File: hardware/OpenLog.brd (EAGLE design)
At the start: 17.8 x 19.1 mm, 20 parts, among them Q1 16MHZ, U1 ATMEGA328P_TQFP, U2 3.3V MIC5205, U3 microSD Socket

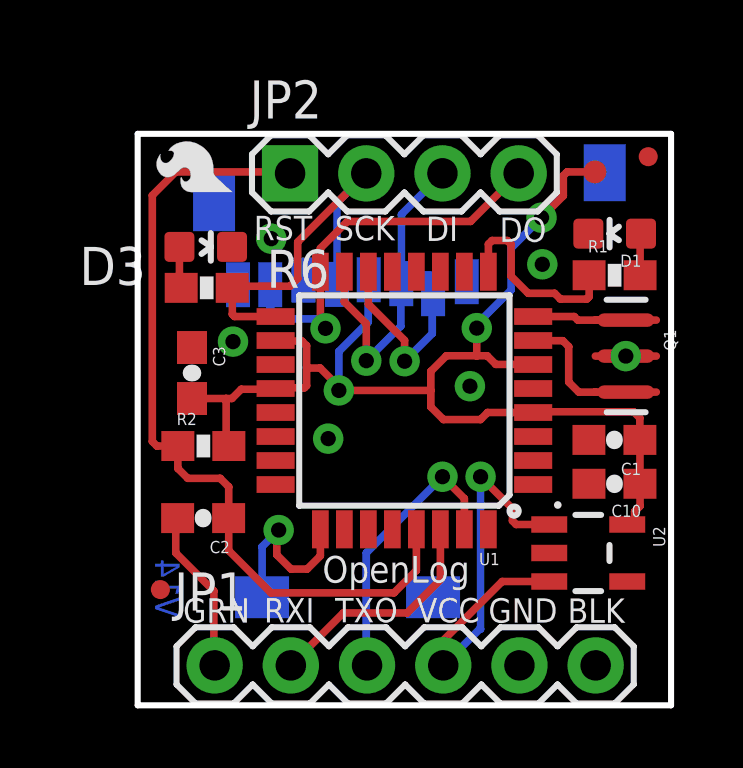
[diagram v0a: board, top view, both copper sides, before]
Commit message: Headers moved on grid.
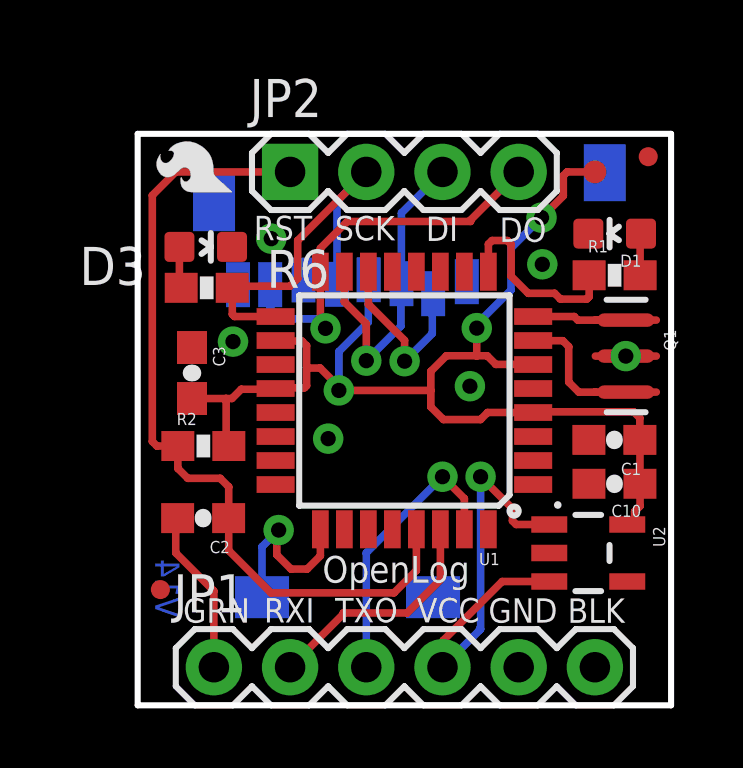
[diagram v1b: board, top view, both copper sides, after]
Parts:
- moved JP1 0.07 mm to (21.6, -8.89)
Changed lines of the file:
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@@
 <setting verticaltext="up"/>
 </settings>
-<grid distance="0.05" unitdist="inch" unit="inch" style="lines" multiple="1" display="yes" altdistance="0.0001" altunitdist="inch" altunit="inch"/>
+<grid distance="0.05" unitdist="inch" unit="inch" style="lines" multiple="1" display="yes" altdistance="0.005" altunitdist="inch" altunit="inch"/>
 <layers>
 <layer number="1" name="Top" color="4" fill="1" visible="yes" active="yes"/>
@@
 <layer number="47" name="Measures" color="7" fill="1" visible="no" active="yes"/>
 <layer number="48" name="Document" color="7" fill="1" visible="no" active="yes"/>
-<layer number="49" name="Reference" color="7" fill="1" visible="yes" active="yes"/>
+<layer number="49" name="Reference" color="7" fill="1" visible="no" active="yes"/>
 <layer number="50" name="dxf" color="7" fill="1" visible="no" active="yes"/>
 <layer number="51" name="tDocu" color="6" fill="1" visible="yes" active="yes"/>
@@
 <attribute name="PROD_ID" value="XTAL-08900" x="35.321240625" y="1.48081875" size="1.778" layer="27" rot="R270" display="off"/>
 </element>
-<element name="JP1" library="SparkFun" package="1X06" value="Serial Connection" x="21.6154" y="-8.8290375"/>
+<element name="JP1" library="SparkFun" package="1X06" value="Serial Connection" x="21.59" y="-8.89"/>
 <element name="C2" library="SparkFun-Capacitors" package="0603-CAP" value="0.1uF" x="21.231859375" y="-3.919221875" rot="R180">
 <attribute name="PROD_ID" value="CAP-00810" x="21.231859375" y="-3.919221875" size="1.778" layer="27" rot="R180" display="off"/>
@@
 <attribute name="VALUE" value="1.0uF" x="34.9402375" y="-1.313175" size="1.778" layer="27" rot="R180" display="off"/>
 </element>
-<element name="JP2" library="SparkFun" package="1X04" value="" x="24.13" y="7.571740625"/>
+<element name="JP2" library="SparkFun" package="1X04" value="" x="24.13" y="7.62"/>
 <element name="U1" library="SparkFun-DigitalIC" package="TQFP32-08" value="ATMEGA328P_TQFP" x="27.94" y="0" rot="R180">
 <attribute name="PROD_ID" value="IC-09069" x="27.94" y="0" size="0.8128" layer="27" font="vector" ratio="15" rot="R180" display="off"/>
@@
 <contactref element="U1" pad="17"/>
 <wire x1="22.204678125" y1="3.753225" x2="22.201240625" y2="3.7566625" width="0.254" layer="1"/>
-<wire x1="25.69464375" y1="3.870953125" x2="25.69464375" y2="6.596384375" width="0.254" layer="16"/>
-<wire x1="25.69464375" y1="6.596384375" x2="26.67" y2="7.571740625" width="0.254" layer="16"/>
-<wire x1="24.384" y1="4.064" x2="24.384" y2="5.285740625" width="0.254" layer="1"/>
-<wire x1="24.384" y1="5.285740625" x2="26.67" y2="7.571740625" width="0.254" layer="1"/>
+<wire x1="25.69464375" y1="3.870953125" x2="25.69464375" y2="6.64464375" width="0.254" layer="16"/>
+<wire x1="24.384" y1="4.064" x2="24.384" y2="5.334" width="0.254" layer="1"/>
 <wire x1="23.6474" y1="2.8" x2="22.2799625" y2="2.8" width="0.254" layer="1"/>
 <wire x1="22.2799625" y1="2.8" x2="22.20468125" y2="2.87528125" width="0.254" layer="1"/>
@@
 <wire x1="24.13" y1="3.81" x2="22.254578125" y2="3.81" width="0.254" layer="1"/>
 <wire x1="22.254578125" y1="3.81" x2="22.201240625" y2="3.7566625" width="0.254" layer="1"/>
+<wire x1="24.384" y1="5.334" x2="26.67" y2="7.62" width="0.254" layer="1"/>
+<wire x1="25.69464375" y1="6.64464375" x2="26.67" y2="7.62" width="0.254" layer="16"/>
 </signal>
 <signal name="MISO">
@@
 <contactref element="U1" pad="16"/>
 <wire x1="25.14" y1="5.074" x2="25.14" y2="4.2926" width="0.254" layer="1"/>
-<wire x1="30.147259375" y1="5.969" x2="31.75" y2="7.571740625" width="0.254" layer="1"/>
 <wire x1="23.45181875" y1="3.086103125" x2="23.815040625" y2="2.72288125" width="0.254" layer="16"/>
 <wire x1="23.815040625" y1="2.72288125" x2="24.99360625" y2="2.72288125" width="0.254" layer="16"/>
@@
 <wire x1="23.45181875" y1="3.086103125" x2="23.45181875" y2="3.846415625" width="0.254" layer="16"/>
 <wire x1="23.45181875" y1="3.846415625" x2="23.4672125" y2="3.861809375" width="0.254" layer="16"/>
+<wire x1="30.147259375" y1="5.969" x2="30.147259375" y2="6.017259375" width="0.254" layer="1"/>
+<wire x1="30.147259375" y1="6.017259375" x2="31.75" y2="7.62" width="0.254" layer="1"/>
 </signal>
 <signal name="MOSI">
@@
 <wire x1="27.82149375" y1="2.479915625" x2="27.82149375" y2="3.876034375" width="0.254" layer="16"/>
 <wire x1="27.82149375" y1="3.876034375" x2="27.8418125" y2="3.896353125" width="0.254" layer="16"/>
-<wire x1="27.8418125" y1="3.896353125" x2="27.8418125" y2="6.203553125" width="0.254" layer="16"/>
-<wire x1="27.8418125" y1="6.203553125" x2="29.21" y2="7.571740625" width="0.254" layer="16"/>
+<wire x1="27.8418125" y1="3.896353125" x2="27.8418125" y2="6.2518125" width="0.254" layer="16"/>
+<wire x1="27.8418125" y1="6.2518125" x2="29.21" y2="7.62" width="0.254" layer="16"/>
 </signal>
 <signal name="N$7">
@@
 <contactref element="U1" pad="31"/>
 <wire x1="29.94" y1="-3.27" x2="29.94" y2="-4.2926" width="0.254" layer="1"/>
-<wire x1="26.67" y1="-5.08" x2="26.67" y2="-8.8036375" width="0.254" layer="16"/>
-<wire x1="26.67" y1="-8.8036375" x2="26.6954" y2="-8.8290375" width="0.254" layer="16"/>
+<wire x1="26.67" y1="-5.08" x2="26.67" y2="-8.89" width="0.254" layer="16"/>
 </signal>
 <signal name="RAW" class="1">
@@
 <wire x1="31.54171875" y1="-3.60171875" x2="30.48" y2="-2.54" width="0.254" layer="1"/>
 <wire x1="30.48" y1="-7.62" x2="30.4444375" y2="-7.62" width="0.254" layer="16"/>
-<wire x1="30.4444375" y1="-7.62" x2="29.2354" y2="-8.8290375" width="0.254" layer="16"/>
-<wire x1="29.2354" y1="-8.8290375" x2="29.2354" y2="-7.99591875" width="0.254" layer="1"/>
 <wire x1="29.2354" y1="-7.99591875" x2="31.19881875" y2="-6.0325" width="0.254" layer="1"/>
 <wire x1="31.19881875" y1="-6.0325" x2="32.76888125" y2="-6.0325" width="0.254" layer="1"/>
 <wire x1="32.76888125" y1="-6.0325" x2="32.768921875" y2="-6.032540625" width="0.254" layer="1"/>
+<wire x1="29.2354" y1="-7.99591875" x2="29.2354" y2="-8.8646" width="0.254" layer="1"/>
+<wire x1="29.2354" y1="-8.8646" x2="29.21" y2="-8.89" width="0.254" layer="1"/>
+<wire x1="30.4444375" y1="-7.62" x2="30.4444375" y2="-7.6555625" width="0.254" layer="16"/>
+<wire x1="30.4444375" y1="-7.6555625" x2="29.21" y2="-8.89" width="0.254" layer="16"/>
 </signal>
 <signal name="N$1">
@@
 <wire x1="20.32" y1="-5.08" x2="20.32" y2="-3.98108125" width="0.254" layer="1"/>
 <wire x1="20.32" y1="-3.98108125" x2="20.381859375" y2="-3.919221875" width="0.254" layer="1"/>
-<wire x1="21.59" y1="-6.35" x2="21.59" y2="-8.8036375" width="0.254" layer="1"/>
-<wire x1="21.59" y1="-8.8036375" x2="21.6154" y2="-8.8290375" width="0.254" layer="1"/>
+<wire x1="21.59" y1="-6.35" x2="21.59" y2="-8.89" width="0.254" layer="1"/>
 </signal>
 <signal name="RXI">
@@
 <wire x1="29.14" y1="-5.9780375" x2="28.03651875" y2="-7.08151875" width="0.254" layer="1"/>
 <wire x1="28.03651875" y1="-7.08151875" x2="25.90291875" y2="-7.08151875" width="0.254" layer="1"/>
-<wire x1="25.90291875" y1="-7.08151875" x2="24.1554" y2="-8.8290375" width="0.254" layer="1"/>
+<wire x1="25.90291875" y1="-7.08151875" x2="25.90291875" y2="-7.11708125" width="0.254" layer="1"/>
+<wire x1="25.90291875" y1="-7.11708125" x2="24.13" y2="-8.89" width="0.254" layer="1"/>
 </signal>
 <signal name="RST">
@@
 <wire x1="22.0853" y1="-5.001259375" x2="22.0853" y2="-3.9226625" width="0.254" layer="1"/>
 <wire x1="22.0853" y1="-3.9226625" x2="22.081859375" y2="-3.919221875" width="0.254" layer="1"/>
-<wire x1="20.32" y1="7.62" x2="24.081740625" y2="7.62" width="0.254" layer="1"/>
-<wire x1="24.081740625" y1="7.62" x2="24.13" y2="7.571740625" width="0.254" layer="1"/>
+<wire x1="20.32" y1="7.62" x2="24.13" y2="7.62" width="0.254" layer="1"/>
 <wire x1="20.38948125" y1="-1.51638125" x2="19.69008125" y2="-1.51638125" width="0.254" layer="1"/>
 <wire x1="19.69008125" y1="-1.51638125" x2="19.53768125" y2="-1.36398125" width="0.254" layer="1"/>
